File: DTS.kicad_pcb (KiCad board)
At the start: 2 copper layers, 162.7 x 122 mm, 55 parts, among them J1 Conn_01x02_Pin, J2 Conn_01x06_Pin, J3 Conn_01x02_Pin, J4 Conn_01x06_Pin, SW1 SW_DIP_x01, U1 4081, U10 4071, U11 4081, U12 4081, U13 4071, U14 4069, U15 4081, U16 4081, U17 4071, U18 4069, U19 4081, U2 4081, U20 4081, U21 4071, U22 4069, U23 4081, U24 4081, U25 4081, U26 4071, U27 4069, U28 4081, U29 4081, U3 4071, U30 4081, U31 4071, U32 4069, U34 4081, U35 4081, U36 4071, U37 4069, U38 4081, U39 4081, U4 4069, U40 4071, U41 4081, U42 4081, U43 4071, U44 4081, U45 4081, U46 4071, U47 4081, U48 4081, U49 LM7805_TO220, U5 4069, U6 4081, U7 4081, U8 4071, U9 4069

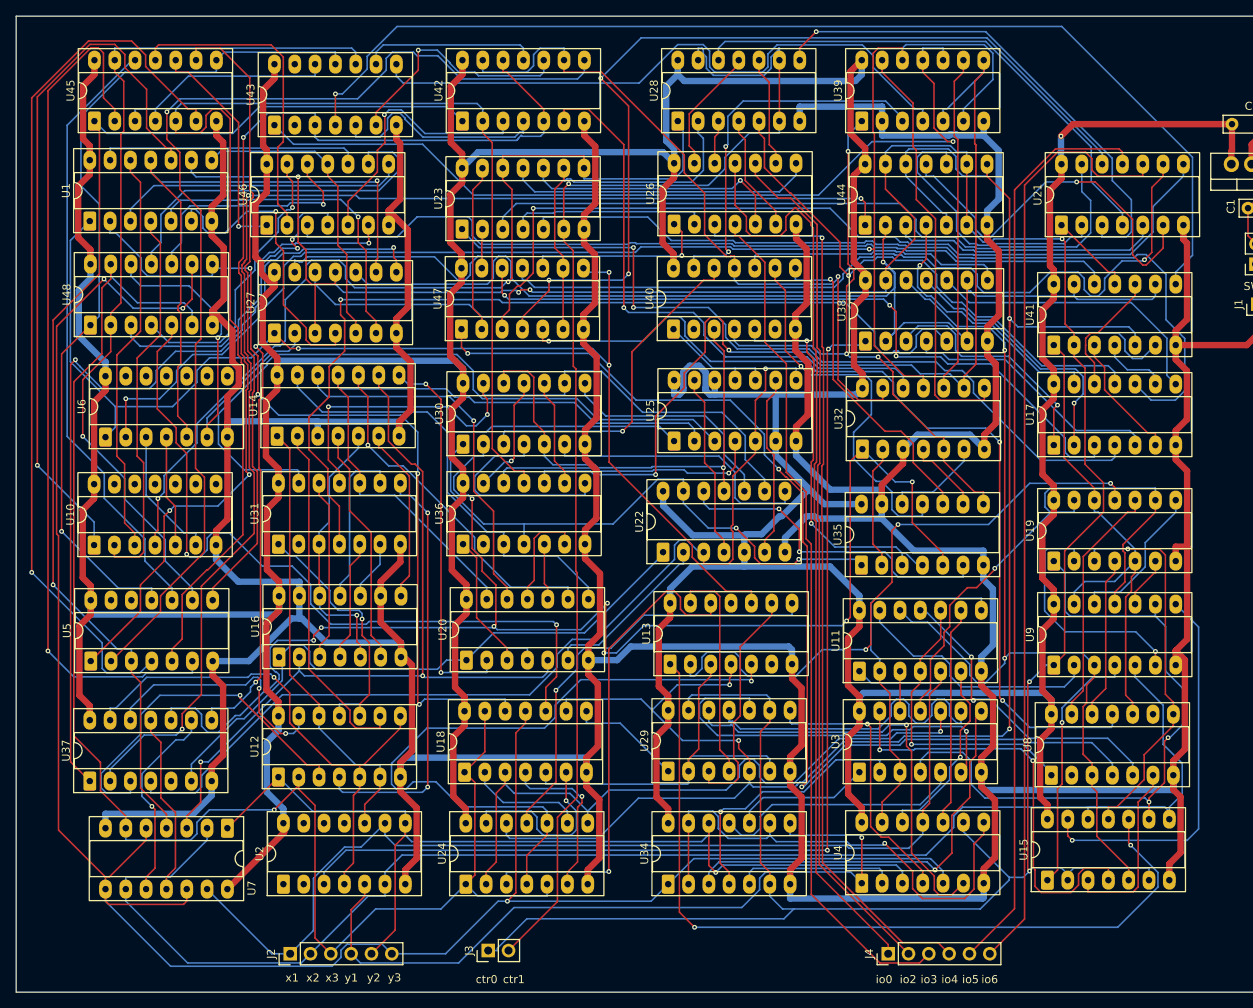
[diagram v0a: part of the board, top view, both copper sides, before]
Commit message: Add files via upload
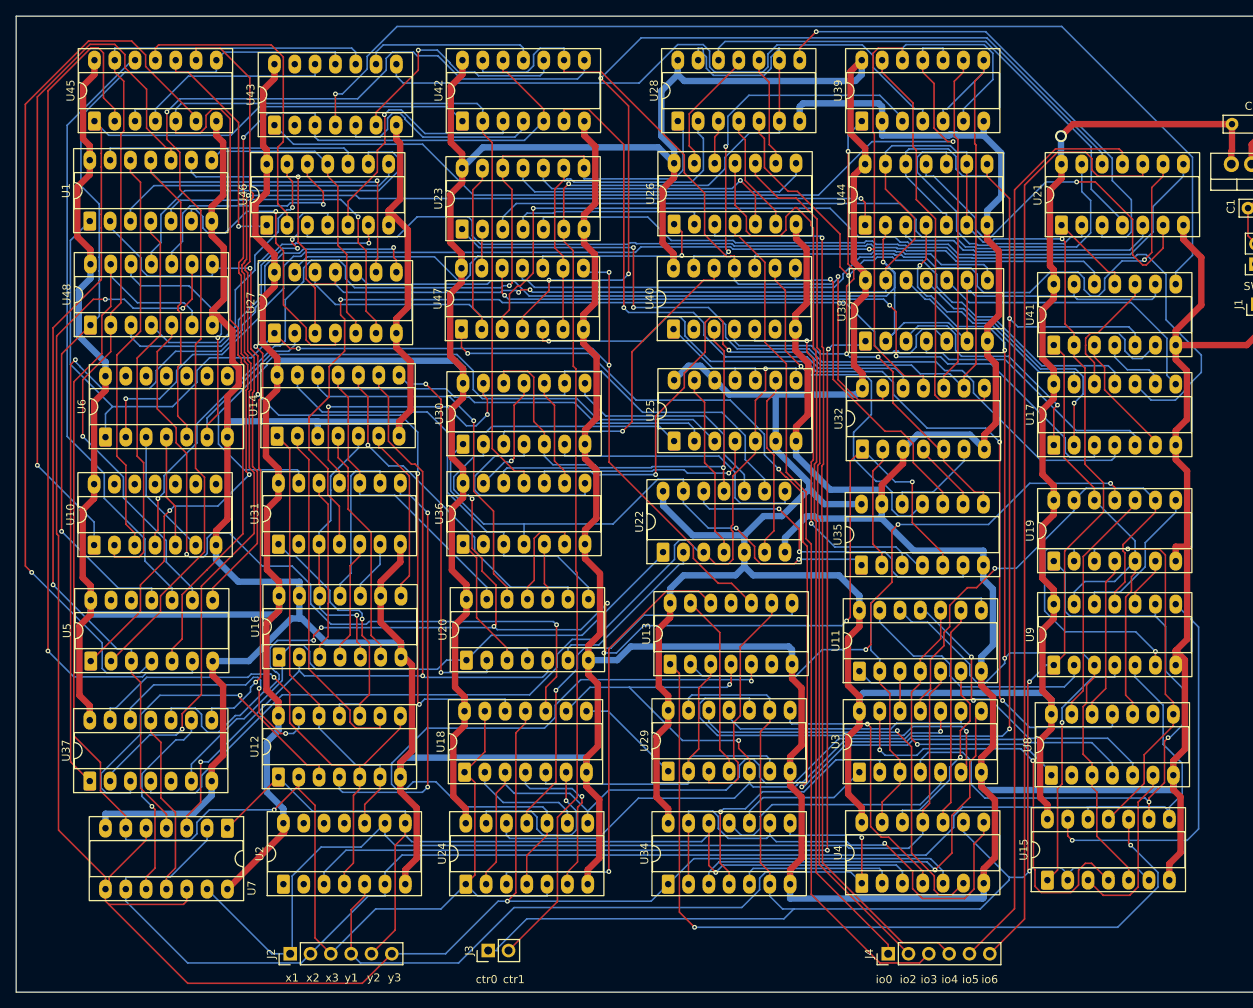
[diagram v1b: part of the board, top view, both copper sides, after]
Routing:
- net /Multiplexer_3b/temp6: track 41.0 -> 32.3 mm
- net VCC: track 808.2 -> 801.2 mm
- net /FullAdder/c_out: track 70.3 -> 63.3 mm
- net /FullAdder1/temp3: track 77.3 -> 72.3 mm
- net /Multiplexer_6b1/(ctrl)': track 142.3 -> 137.3 mm
- net /FullAdder2/temp3: track 27.8 -> 23.0 mm
- net y3: track 264.1 -> 260.7 mm
- net /FullAdder2/xy: track 61.5 -> 58.5 mm
- net GND: track 855.8 -> 857.9 mm
- net xor3: track 231.8 -> 233.8 mm
- net /y3': track 53.8 -> 52.0 mm
- net x1: track 139.9 -> 141.6 mm
- net /Multiplexer_6b1/iout_2: track 106.1 -> 107.9 mm
- net /Multiplier/FullAdder4/xy' + x'y: track 131.8 -> 130.8 mm
- net /Multiplier/(A2B1)': track 123.0 -> 122.1 mm
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
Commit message: Add files via upload
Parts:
- added D1: LED, Connector_PinHeader_2.54mm:PinHeader_1x02_P2.54mm_Vertical, F.Cu at (204.2, 38.2)
- added D10: LED, Connector_PinHeader_2.54mm:PinHeader_1x02_P2.54mm_Vertical, F.Cu at (199.0, 146.9)
- added D11: LED, Connector_PinHeader_2.54mm:PinHeader_1x02_P2.54mm_Vertical, F.Cu at (199.0, 142.4)
- added D12: LED, Connector_PinHeader_2.54mm:PinHeader_1x02_P2.54mm_Vertical, F.Cu at (199.0, 137.8)
- added D13: LED, Connector_PinHeader_2.54mm:PinHeader_1x02_P2.54mm_Vertical, F.Cu at (199.0, 133.2)
- added D14: LED, Connector_PinHeader_2.54mm:PinHeader_1x02_P2.54mm_Vertical, F.Cu at (199.0, 128.6)
- added D15: LED, Connector_PinHeader_2.54mm:PinHeader_1x02_P2.54mm_Vertical, F.Cu at (199.0, 124.0)
- added D2: LED, Connector_PinHeader_2.54mm:PinHeader_1x02_P2.54mm_Vertical, F.Cu at (67.0, 73.0)
- added D3: LED, Connector_PinHeader_2.54mm:PinHeader_1x02_P2.54mm_Vertical, F.Cu at (71.5, 73.0)
- added D4: LED, Connector_PinHeader_2.54mm:PinHeader_1x02_P2.54mm_Vertical, F.Cu at (76.0, 73.0)
- added D5: LED, Connector_PinHeader_2.54mm:PinHeader_1x02_P2.54mm_Vertical, F.Cu at (76.0, 88.0)
- added D6: LED, Connector_PinHeader_2.54mm:PinHeader_1x02_P2.54mm_Vertical, F.Cu at (71.5, 88.0)
- added D7: LED, Connector_PinHeader_2.54mm:PinHeader_1x02_P2.54mm_Vertical, F.Cu at (67.0, 88.0)
- added D8: LED, Connector_PinHeader_2.54mm:PinHeader_1x02_P2.54mm_Vertical, F.Cu at (67.0, 61.0)
- added D9: LED, Connector_PinHeader_2.54mm:PinHeader_1x02_P2.54mm_Vertical, F.Cu at (79.0, 63.5)
- added R1: R, Connector_PinHeader_2.54mm:PinHeader_1x02_P2.54mm_Vertical, F.Cu at (67.0, 78.0)
- added R10: R, Connector_PinHeader_2.54mm:PinHeader_1x02_P2.54mm_Vertical, F.Cu at (207.0, 142.5)
- added R11: R, Connector_PinHeader_2.54mm:PinHeader_1x02_P2.54mm_Vertical, F.Cu at (207.0, 137.9)
- added R12: R, Connector_PinHeader_2.54mm:PinHeader_1x02_P2.54mm_Vertical, F.Cu at (207.0, 133.3)
- added R13: R, Connector_PinHeader_2.54mm:PinHeader_1x02_P2.54mm_Vertical, F.Cu at (207.0, 128.7)
- added R14: R, Connector_PinHeader_2.54mm:PinHeader_1x02_P2.54mm_Vertical, F.Cu at (207.0, 124.1)
- added R2: R, Connector_PinHeader_2.54mm:PinHeader_1x02_P2.54mm_Vertical, F.Cu at (71.5, 78.0)
- added R3: R, Connector_PinHeader_2.54mm:PinHeader_1x02_P2.54mm_Vertical, F.Cu at (76.0, 78.0)
- added R4: R, Connector_PinHeader_2.54mm:PinHeader_1x02_P2.54mm_Vertical, F.Cu at (76.0, 93.0)
- added R5: R, Connector_PinHeader_2.54mm:PinHeader_1x02_P2.54mm_Vertical, F.Cu at (71.5, 93.0)
- added R6: R, Connector_PinHeader_2.54mm:PinHeader_1x02_P2.54mm_Vertical, F.Cu at (67.0, 93.0)
- added R7: R, Connector_PinHeader_2.54mm:PinHeader_1x02_P2.54mm_Vertical, F.Cu at (71.0, 61.0)
- added R8: R, Connector_PinHeader_2.54mm:PinHeader_1x02_P2.54mm_Vertical, F.Cu at (83.0, 63.5)
- added R9: R, Connector_PinHeader_2.54mm:PinHeader_1x02_P2.54mm_Vertical, F.Cu at (207.0, 147.0)
- added SW2: SW_DIP_x01, Connector_PinHeader_2.54mm:PinHeader_1x03_P2.54mm_Vertical, F.Cu at (81.0, 70.5)
- added SW3: SW_DIP_x01, Connector_PinHeader_2.54mm:PinHeader_1x03_P2.54mm_Vertical, F.Cu at (85.0, 70.5)
- added SW4: SW_DIP_x01, Connector_PinHeader_2.54mm:PinHeader_1x03_P2.54mm_Vertical, F.Cu at (85.0, 80.5)
- added SW5: SW_DIP_x01, Connector_PinHeader_2.54mm:PinHeader_1x03_P2.54mm_Vertical, F.Cu at (81.0, 89.9)
- added SW6: SW_DIP_x01, Connector_PinHeader_2.54mm:PinHeader_1x03_P2.54mm_Vertical, F.Cu at (81.0, 80.5)
- added SW7: SW_DIP_x01, Connector_PinHeader_2.54mm:PinHeader_1x03_P2.54mm_Vertical, F.Cu at (85.0, 89.9)
- added SW8: SW_DIP_x01, Connector_PinHeader_2.54mm:PinHeader_1x03_P2.54mm_Vertical, F.Cu at (75.0, 60.4)
- added SW9: SW_DIP_x01, Connector_PinHeader_2.54mm:PinHeader_1x03_P2.54mm_Vertical, F.Cu at (87.0, 60.5)
- C1, C2: footprint Capacitor_THT:C_Rect_L7.0mm_W2.0mm_P5.00mm -> Capacitor_THT:C_Radial_D6.3mm_H5.0mm_P2.50mm
- SW1: footprint Connector_PinSocket_2.54mm:PinSocket_1x02_P2.54mm_Vertical -> Connector_PinHeader_2.54mm:PinHeader_1x03_P2.54mm_Vertical
- moved U15 140.0 mm to (71.1, 54.1), turned to 180 degrees
- moved U1 136.5 mm to (179.9, 127.3), turned to 0 degrees
- moved U5 127.4 mm to (182.9, 61.8), turned to 0 degrees
- moved U45 125.2 mm to (183.4, 82.8), turned to 0 degrees
- moved U27 124.2 mm to (201.0, 119.1), turned to 180 degrees
- moved U8 122.6 mm to (83.4, 54.5), turned to 180 degrees
- moved U48 121.1 mm to (174.5, 118.2), turned to 180 degrees
- moved U10 118.8 mm to (174.0, 142.2), turned to 180 degrees
- moved U6 116.6 mm to (180.9, 103.8), turned to 0 degrees
- moved U39 105.7 mm to (75.5, 103.8), turned to 0 degrees
- moved U9 105.3 mm to (91.8, 60.9), turned to 0 degrees
- moved U3 101.1 mm to (61.5, 103.8), turned to 0 degrees
- moved U46 100.7 mm to (177.5, 98.1), turned to 180 degrees
- moved U19 98.8 mm to (95.9, 54.1), turned to 180 degrees
- moved J3 97.7 mm to (61.5, 63.3), turned to 180 degrees
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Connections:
- net /Multiplexer_6b1/i0_0 renamed /mult0
- net /Multiplexer_6b1/i0_1 renamed /mult1
- net /Multiplexer_6b1/i0_2 renamed /mult2
- net /Multiplexer_6b1/i0_3 renamed /mult3
- net /Multiplexer_6b1/i0_4 renamed /mult4
- net /Multiplexer_6b1/i0_5 renamed /mult5
- net /Multiplexer_6b2/iout_0 renamed /output 0
- net /Multiplexer_6b2/iout_1 renamed /output 1
- net /Multiplexer_6b2/iout_2 renamed /output 2
- net /Multiplexer_6b2/iout_3 renamed /output 3
- net /Multiplexer_6b2/iout_4 renamed /output 4
- net /Multiplexer_6b2/iout_5 renamed /output 5
- J2 pad 1: x1 -> x0
- J2 pad 2: x2 -> x1
- J2 pad 3: x3 -> x2
- J2 pad 4: y1 -> y0
- J2 pad 5: y2 -> y1
- J2 pad 6: y3 -> y2
- U1 pad 1: s3 -> s2
- U11 pad 1: x1 -> x0
- U11 pad 10: /FullAdder/xy' -> /FullAdder/x'y
- U11 pad 12: xor1 -> xor0
- U11 pad 2: /y_signed1 -> /y_signed0
- U11 pad 5: x1 -> x0
- U11 pad 8: /y_signed1 -> /y_signed0
- U12 pad 1: y2 -> y1
- U12 pad 11: /Multiplier/FullAdder/xy' -> /Multiplier/FullAdder/x'y
- U12 pad 2: x3 -> x2
- U13 pad 10: s3 -> s2
- U13 pad 4: xor3 -> xor2
- U15 pad 12: x2 -> x1
- U15 pad 5: xor1 -> xor0
- U15 pad 8: x2 -> x1
- U15 pad 9: /y_signed2 -> /y_signed1
- U18 pad 1: x3 -> x2
- U18 pad 11: y3 -> y2
- U18 pad 13: x3 -> x2
- U18 pad 3: /y_signed3 -> /y_signed2
- U18 pad 9: xor3 -> xor2
- U19 pad 1: /y_signed2 -> /y_signed1
- U19 pad 12: xor2 -> xor1
- U19 pad 3: /FullAdder1/xy' -> /FullAdder1/x'y
- U19 pad 5: xor2 -> xor1
- U2 pad 5: y1 -> y0
- U2 pad 6: x2 -> x1
- U2 pad 8: y2 -> y1
- U2 pad 9: x1 -> x0
- U20 pad 4: /Multiplier/FullAdder1/xy' -> /Multiplier/FullAdder1/x'y
- U24 pad 1: x3 -> x2
- U24 pad 10: /FullAdder2/xy' -> /FullAdder2/x'y
- U24 pad 12: xor3 -> xor2
- U24 pad 2: /y_signed3 -> /y_signed2
- U24 pad 5: x3 -> x2
- U24 pad 8: /y_signed3 -> /y_signed2
- U25 pad 11: /Multiplier/FullAdder2/xy' -> /Multiplier/FullAdder2/x'y
- U27 pad 1: s3 -> s2
- U29 pad 12: /y3' -> /y2'
- U29 pad 5: xor3 -> xor2
- U29 pad 8: /y2' -> /y1'
- U3 pad 10: /y_signed3 -> /y_signed2
- U3 pad 3: /y_signed1 -> /y_signed0
- U3 pad 4: /y_signed2 -> /y_signed1
- U34 pad 1: y3 -> y2
- U34 pad 12: y2 -> y1
- U34 pad 5: /y1' -> /y0'
- U34 pad 8: y1 -> y0
- U35 pad 4: /Multiplier/FullAdder3/xy' -> /Multiplier/FullAdder3/x'y
- U38 pad 12: xor1 -> xor0
- U39 pad 11: /Multiplier/FullAdder4/xy' -> /Multiplier/FullAdder4/x'y
- U4 pad 1: y1 -> y0
- U4 pad 11: x1 -> x0
- U4 pad 13: /y_signed1 -> /y_signed0
- U4 pad 2: /y1' -> /y0'
- U4 pad 3: y2 -> y1
- U4 pad 4: /y2' -> /y1'
- U4 pad 5: y3 -> y2
- U4 pad 6: /y3' -> /y2'
- U41 pad 1: xor2 -> xor1
- U41 pad 5: xor3 -> xor2
- U44 pad 12: xor3 -> xor2
- U44 pad 5: xor3 -> xor2
- U44 pad 8: xor3 -> xor2
- U45 pad 4: /Multiplier/FullAdder5/xy' -> /Multiplier/FullAdder5/x'y
- U47 pad 1: s1 -> s0
- U47 pad 5: s2 -> s1
- U47 pad 8: s3 -> s2
- U48 pad 13: x3 -> x2
- U48 pad 6: x3 -> x2
- U48 pad 9: y3 -> y2
- U6 pad 1: s3 -> s2
- U7 pad 1: y2 -> y1
- U7 pad 12: y3 -> y2
- U7 pad 13: x1 -> x0
- U7 pad 2: x2 -> x1
- U7 pad 5: y3 -> y2
- U7 pad 6: x3 -> x2
- U7 pad 8: y3 -> y2
- U7 pad 9: x2 -> x1
- U8 pad 10: xor2 -> xor1
- U8 pad 11: s2 -> s1
- U8 pad 3: xor1 -> xor0
- U8 pad 4: s1 -> s0
- U9 pad 13: xor2 -> xor1
- U9 pad 3: xor1 -> xor0
- U9 pad 5: x2 -> x1
- U9 pad 9: /y_signed2 -> /y_signed1
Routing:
- net GND: track 857.9 -> 71.1 mm
- net VCC: track 801.2 -> 40.1 mm, vias 1 -> 0
- net ctrl_out0: track 403.9 -> 0.00 mm, vias 6 -> 0
- net y3: track 260.7 -> 0.00 mm, vias 3 -> 0
- net xor3: track 233.8 -> 0.00 mm, vias 4 -> 0
- net /Multiplier/(A1B2)': track 212.7 -> 0.00 mm, vias 3 -> 0
- net ctrl_out1: track 204.7 -> 0.00 mm, vias 1 -> 0
- net x3: track 196.3 -> 0.00 mm, vias 1 -> 0
- net /Multiplier/(A0B2)': track 178.1 -> 0.00 mm, vias 8 -> 0
- net /Multiplier/cout3: track 173.3 -> 0.00 mm
- net /mult5: track 164.0 -> 0.00 mm, vias 3 -> 0
- net s3: track 151.5 -> 0.00 mm, vias 3 -> 0
- net /Multiplier/A2B2: track 146.2 -> 0.00 mm, vias 1 -> 0
- net /mult3: track 139.0 -> 0.00 mm, vias 1 -> 0
- net /Multiplexer_6b1/(ctrl)': track 137.3 -> 0.00 mm, vias 1 -> 0
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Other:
- board size 162.7 x 122 mm -> 162.5 x 123 mm
- board text added: "POWER IN"
- board text removed: "ctr0"
- board text removed: "ctr1"
- board text removed: "io0"
- board text removed: "io2"
- board text removed: "io3"
- board text removed: "io4"
- board text removed: "io5"
- board text removed: "io6"
- board text removed: "x1"
- board text removed: "x2"
- board text removed: "x3"
- board text removed: "y1"
- board text removed: "y2"
- board text removed: "y3"

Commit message: Add files via upload
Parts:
- added G***: LOGO, LOGO, F.Cu at (204.0, 82.5)
- moved U24 127.2 mm to (168.0, 57.3)
- moved U13 122.2 mm to (155.8, 34.7), turned to 0 degrees
- moved U1 112.3 mm to (67.6, 126.1)
- moved U34 108.2 mm to (67.2, 34.7), turned to 0 degrees
- moved U6 102.9 mm to (80.4, 126.2)
- moved U5 99.4 mm to (92.6, 103.3)
- moved U15 99.0 mm to (168.2, 34.7), turned to 0 degrees
- moved U36 98.7 mm to (80.0, 103.4)
- moved U27 95.9 mm to (105.4, 126.6), turned to 0 degrees
- moved U43 91.9 mm to (117.6, 103.5)
- moved U42 90.8 mm to (105.2, 103.4)
- moved U19 88.4 mm to (182.0, 34.3), turned to 0 degrees
- moved U25 87.0 mm to (67.4, 103.7)
- moved U39 83.5 mm to (155.8, 81.0)
- moved U17 83.2 mm to (196.4, 104.3), turned to 0 degrees
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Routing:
- net GND: track 71.1 -> 904.7 mm
- net VCC: track 40.1 -> 806.8 mm
- net ctrl_out0: track 0.00 -> 419.5 mm, vias 0 -> 6
- net ctrl_out1: track 0.00 -> 271.3 mm, vias 0 -> 3
- net y2: track 38.7 -> 308.1 mm, vias 0 -> 5
- net s2: track 0.00 -> 257.0 mm, vias 0 -> 6
- net xor2: track 0.00 -> 219.4 mm, vias 0 -> 2
- net /Signed_Extended/A2': track 0.00 -> 204.0 mm, vias 0 -> 3
- net x2: track 51.0 -> 251.0 mm, vias 0 -> 2
- net /Signed_Extended/S2': track 0.00 -> 164.5 mm, vias 0 -> 5
- net xor1: track 0.00 -> 162.7 mm, vias 0 -> 4
- net /FullAdder/c_out: track 0.00 -> 162.6 mm, vias 0 -> 6
- net /mult5: track 0.00 -> 154.7 mm, vias 0 -> 4
- net xor0: track 0.00 -> 147.8 mm
- net /Multiplexer_6b2/(ctrl)': track 0.00 -> 147.8 mm, vias 0 -> 3
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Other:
- board size 162.5 x 123 mm -> 157 x 122.5 mm
- board text added: "Duong Phan Quang Bach Nguyen Dac Hai Dang Nguyen Duc Tung Nguyen Doan Hong Thai"
- board text added: "I HOPE THIS WORK :v"
- board text added: "Input LEDs"
- board text added: "Output LEDs"
- board text added: "Select Operation"
- board text added: "ctrl0"
- board text added: "out0"
- board text added: "x0"
- board text added: "y0"

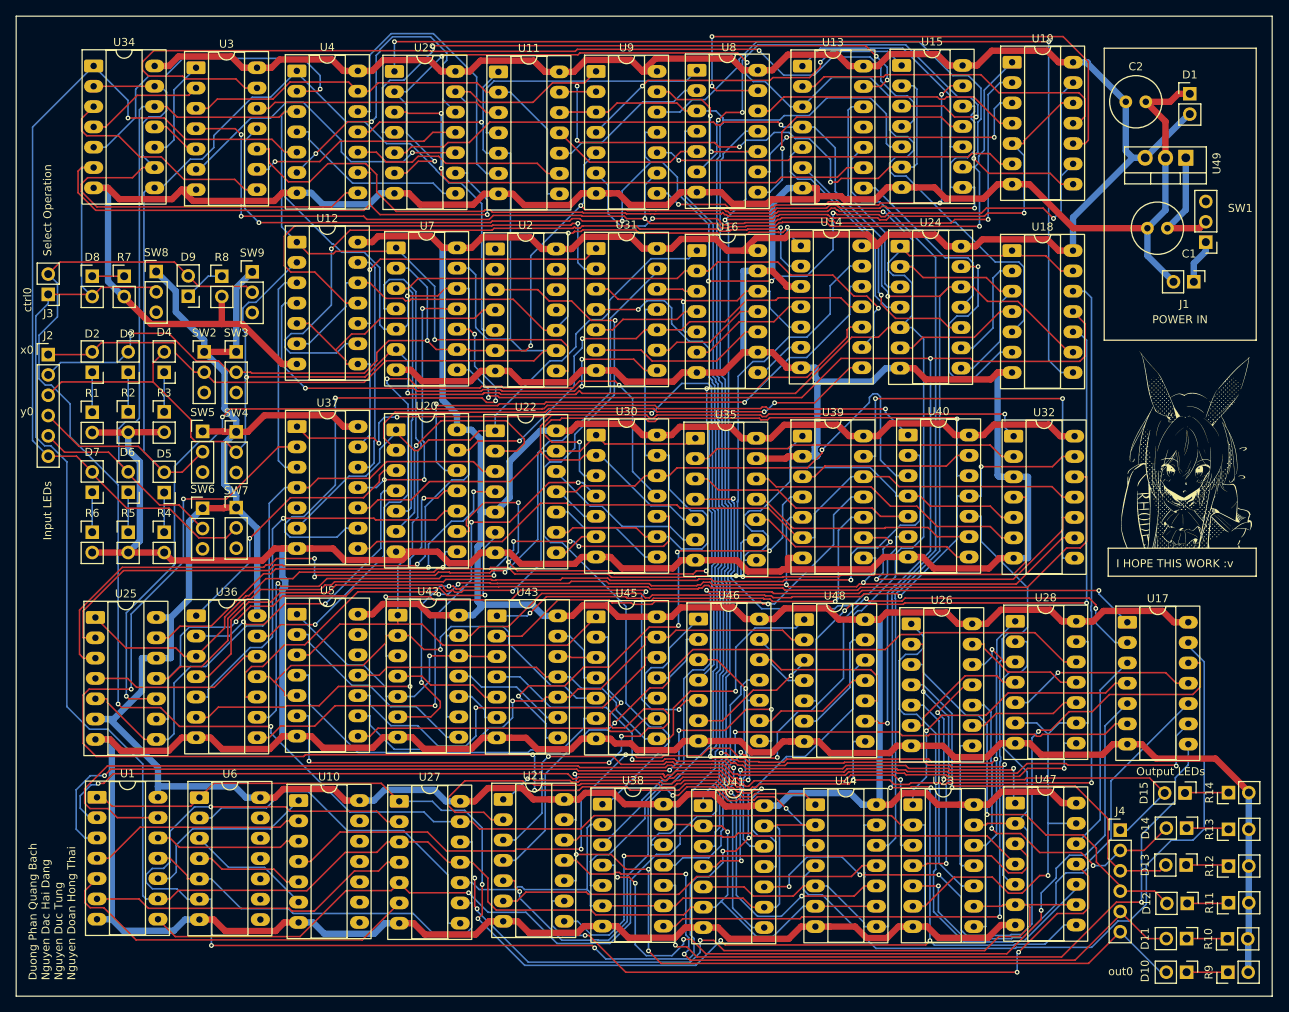
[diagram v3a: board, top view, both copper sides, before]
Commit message: Add files via upload
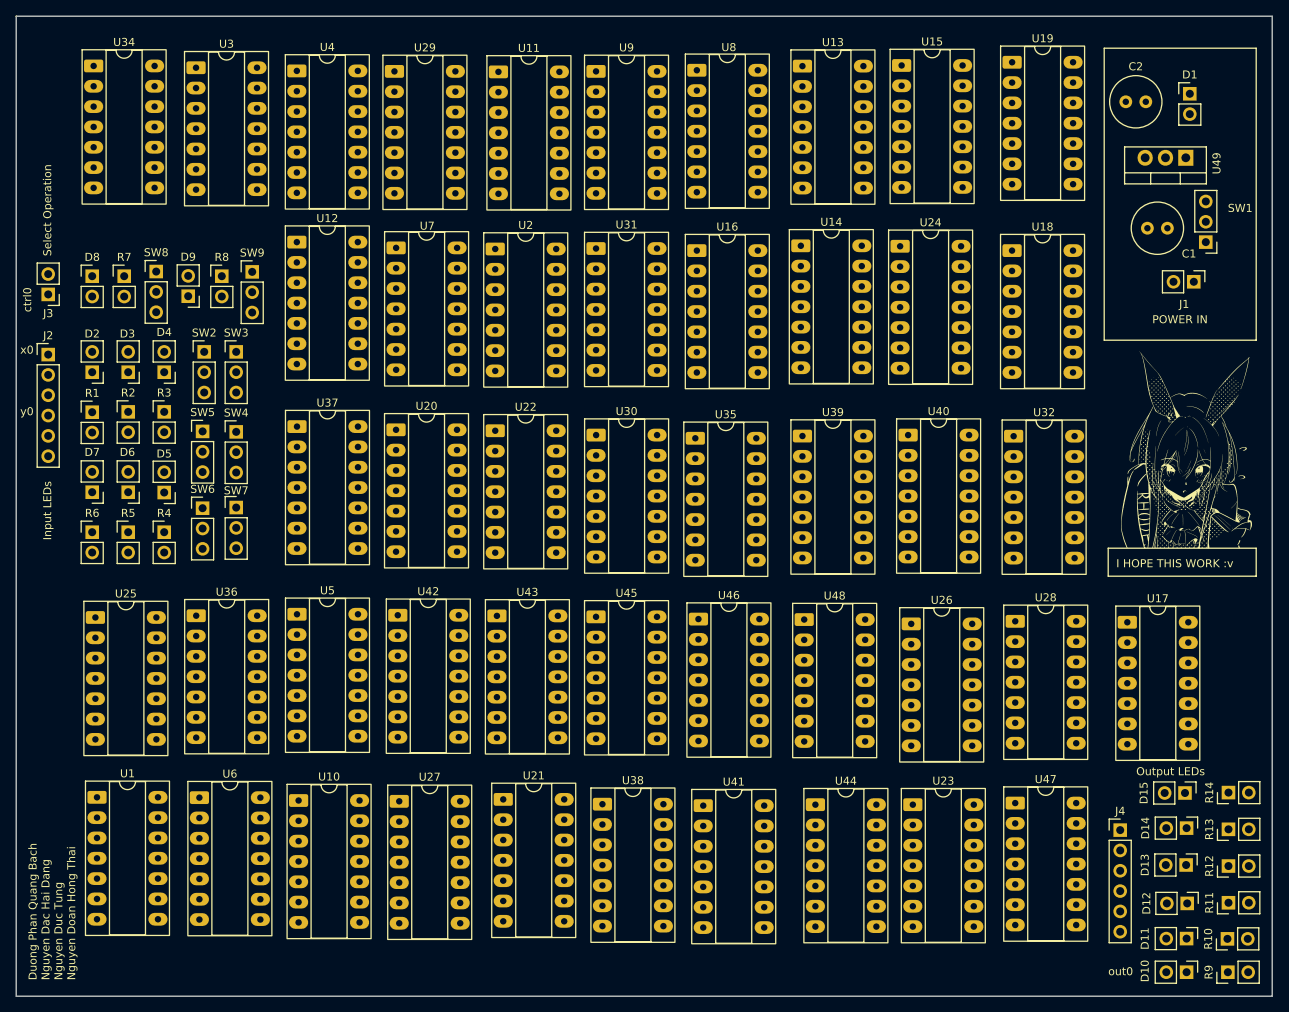
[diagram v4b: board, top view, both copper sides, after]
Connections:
- U19 pad 10: /FullAdder1/temp2 -> unconnected-(U19-Pad10)
- U2 pad 1: unconnected-(U2-Pad1) -> y0
- U2 pad 11: unconnected-(U2-Pad11) -> /Multiplier/A2B0
- U2 pad 12: unconnected-(U2-Pad12) -> y0
- U2 pad 13: unconnected-(U2-Pad13) -> x2
- U2 pad 2: unconnected-(U2-Pad2) -> x0
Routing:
- net GND: track 904.7 -> 0.00 mm
- net VCC: track 806.8 -> 0.00 mm
- net ctrl_out0: track 419.5 -> 0.00 mm, vias 6 -> 0
- net y2: track 308.1 -> 0.00 mm, vias 5 -> 0
- net ctrl_out1: track 271.3 -> 0.00 mm, vias 3 -> 0
- net s2: track 257.0 -> 0.00 mm, vias 6 -> 0
- net x2: track 251.0 -> 0.00 mm, vias 2 -> 0
- net xor2: track 219.4 -> 0.00 mm, vias 2 -> 0
- net /Signed_Extended/A2': track 204.0 -> 0.00 mm, vias 3 -> 0
- net x1: track 178.1 -> 0.00 mm, vias 5 -> 0
- net /Signed_Extended/S2': track 164.5 -> 0.00 mm, vias 5 -> 0
- net xor1: track 162.7 -> 0.00 mm, vias 4 -> 0
- net /FullAdder/c_out: track 162.6 -> 0.00 mm, vias 6 -> 0
- net y1: track 159.6 -> 0.00 mm, vias 1 -> 0
- net /mult5: track 154.7 -> 0.00 mm, vias 4 -> 0
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
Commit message: Add files via upload
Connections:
- U19 pad 10: unconnected-(U19-Pad10) -> /FullAdder1/temp2
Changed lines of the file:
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@@
 			(layers "*.Cu" "*.Mask")
 			(remove_unused_layers no)
-			(net "unconnected-(U19-Pad10)")
+			(net "/FullAdder1/temp2")
 			(pintype "output")
 		)
